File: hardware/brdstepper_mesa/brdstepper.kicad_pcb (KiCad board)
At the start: 4 copper layers, 28 x 28 mm, 88 parts, among them J2 VM / GND / EN, J3 MOTOR, J4 SMART-SERIAL, U1 STM32G473CEU6, U2 DRV8876RGTR, U3 DRV8876RGTR, U4 AS5047P-ATSM, U5 TLV75533PDBVR, U6 TPS560430XDBVR, U8 SN65HVD30DR, Y1 8MHz

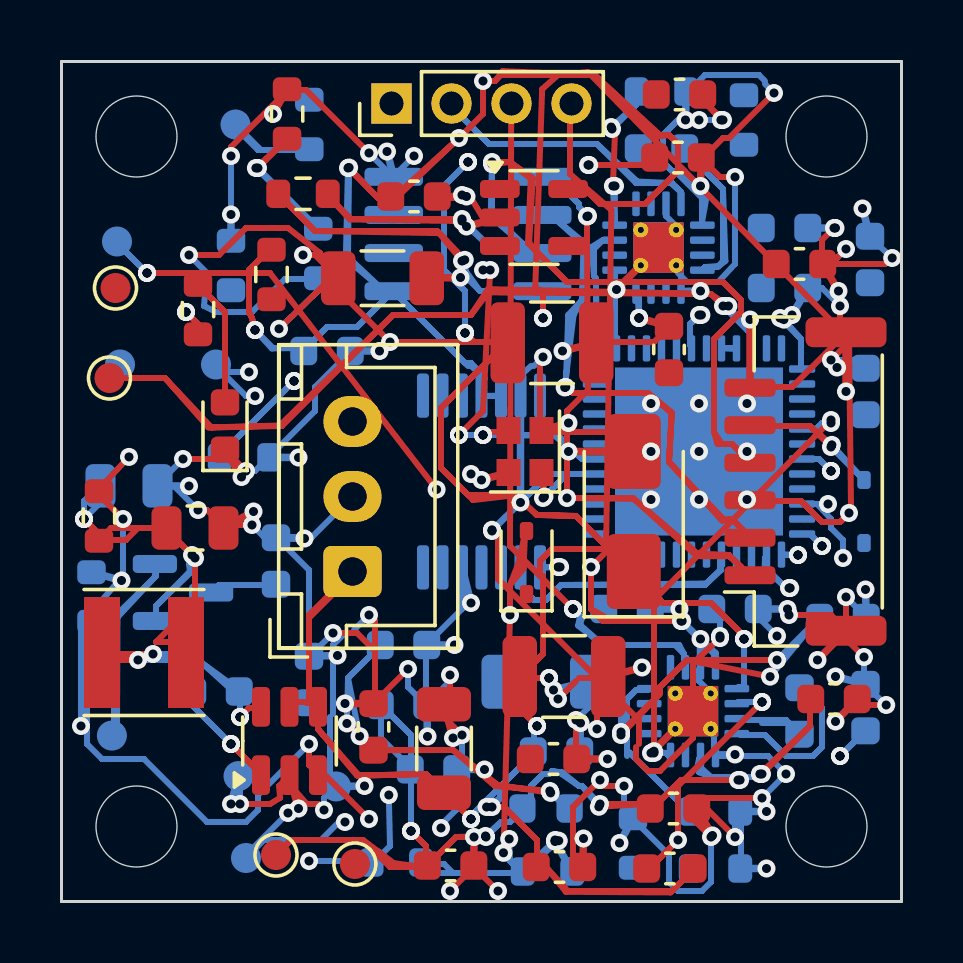
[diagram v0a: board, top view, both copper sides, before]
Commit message: brdstepper: re-placed boards without J2 (routing run in progress)
Both boards re-placed with J2 gone, courtyard gap 0.40 mm. Snapshot taken
while the first plane-aware routing run is still going: copper may be
missing or partial.

Co-Authored-By: Claude Sonnet 5.5 <noreply@anthropic.com>
Claude-Session: https://claude.ai/code/session_017CSpK2B8oMBAmr39Kq1RSC
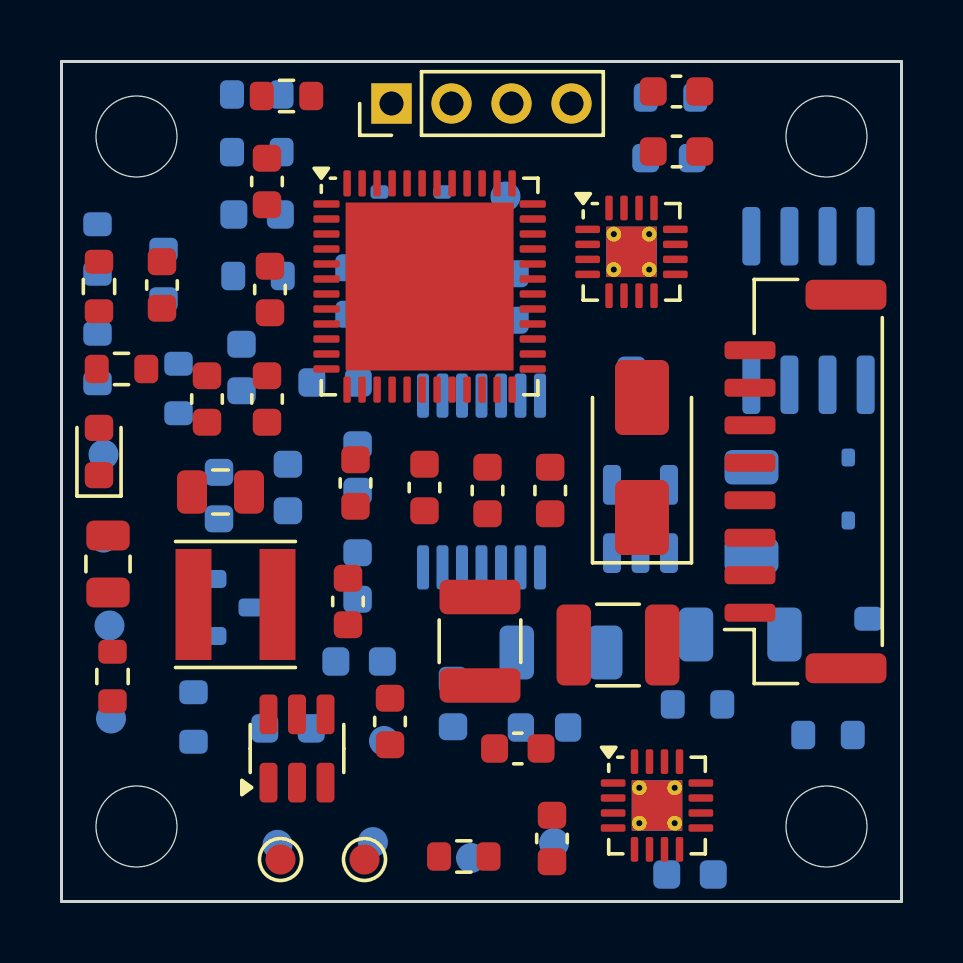
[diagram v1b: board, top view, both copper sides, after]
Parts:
- removed J2: VM / GND / EN, Connector_JST:JST_XH_B3B-XH-A_1x03_P2.50mm_Vertical
- C11, C12, C23, C31, C33, C34, C36, C38, C7, R12, R15, TP6, TP9, U1, U2, U3: moved to F.Cu
- C14, C19, C21, C24, C27, C3, C35, D5, R14, R20, TP11, TP2, TP3, TP4, U5, Y1: moved to B.Cu
- J4: footprint Connector_JST:JST_GH_SM06B-GHS-TB_1x06-1MP_P1.25mm_Horizontal -> Connector_JST:JST_GH_SM08B-GHS-TB_1x08-1MP_P1.25mm_Horizontal
- moved C36 26.6 mm to (92.8, 90.0)
- moved R16 25.9 mm to (92.5, 89.0)
- moved R15 25.8 mm to (93.5, 87.2)
- moved R20 25.1 mm to (111.5, 108.5)
- moved R5 24.0 mm to (89.9, 96.9), turned to 90 degrees
- moved R14 23.4 mm to (112.9, 105.4)
- moved C9 21.6 mm to (89.3, 93.5), turned to 90 degrees
- moved C33 20.1 mm to (101.2, 108.9), turned to 0 degrees
- moved TP3 19.3 mm to (93.2, 112.1)
- moved TP6 18.4 mm to (96.1, 112.6)
- moved C22 17.7 mm to (92.5, 91.1)
- moved C17 17.7 mm to (95.1, 96.7), turned to 0 degrees
- moved R10 17.0 mm to (92.5, 93.2), turned to 0 degrees
- moved C15 16.7 mm to (95.6, 93.7), turned to 90 degrees
- moved C21 16.4 mm to (95.9, 103.2), turned to 90 degrees
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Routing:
- net GND: track 241.0 -> 0.00 mm, vias 109 -> 0
- net VM: track 188.9 -> 0.00 mm, vias 21 -> 0
- net 3V3: track 139.6 -> 0.00 mm, vias 16 -> 0
- net SS_RX+: track 85.3 -> 0.00 mm, vias 5 -> 0
- net SS_RX-: track 58.7 -> 0.00 mm, vias 4 -> 0
- net SWDIO: track 57.4 -> 0.00 mm, vias 6 -> 0
- net EN_IN: track 56.9 -> 0.00 mm, vias 7 -> 0
- net BUCK_FB: track 50.2 -> 0.00 mm, vias 5 -> 0
- net USB_DP: track 50.2 -> 0.00 mm, vias 4 -> 0
- net TP_PB10: track 50.2 -> 0.00 mm, vias 2 -> 0
- net SWCLK: track 48.7 -> 0.00 mm, vias 4 -> 0
- net LED: track 46.9 -> 0.00 mm, vias 4 -> 0
- net COIL_B-: track 45.7 -> 0.00 mm, vias 3 -> 0
- net OSC_IN: track 45.6 -> 0.00 mm, vias 6 -> 0
- net COIL_B+: track 45.5 -> 0.00 mm, vias 2 -> 0
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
